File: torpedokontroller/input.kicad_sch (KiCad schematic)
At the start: 33 parts, among them IC8 TCAN3414DR, J2 653104124022, J8 USB_C_Receptacle_USB2.0_16P, U10 173950336, U4 WE-TVS-82400102, U8 BME280, U9 TPS26400PWP

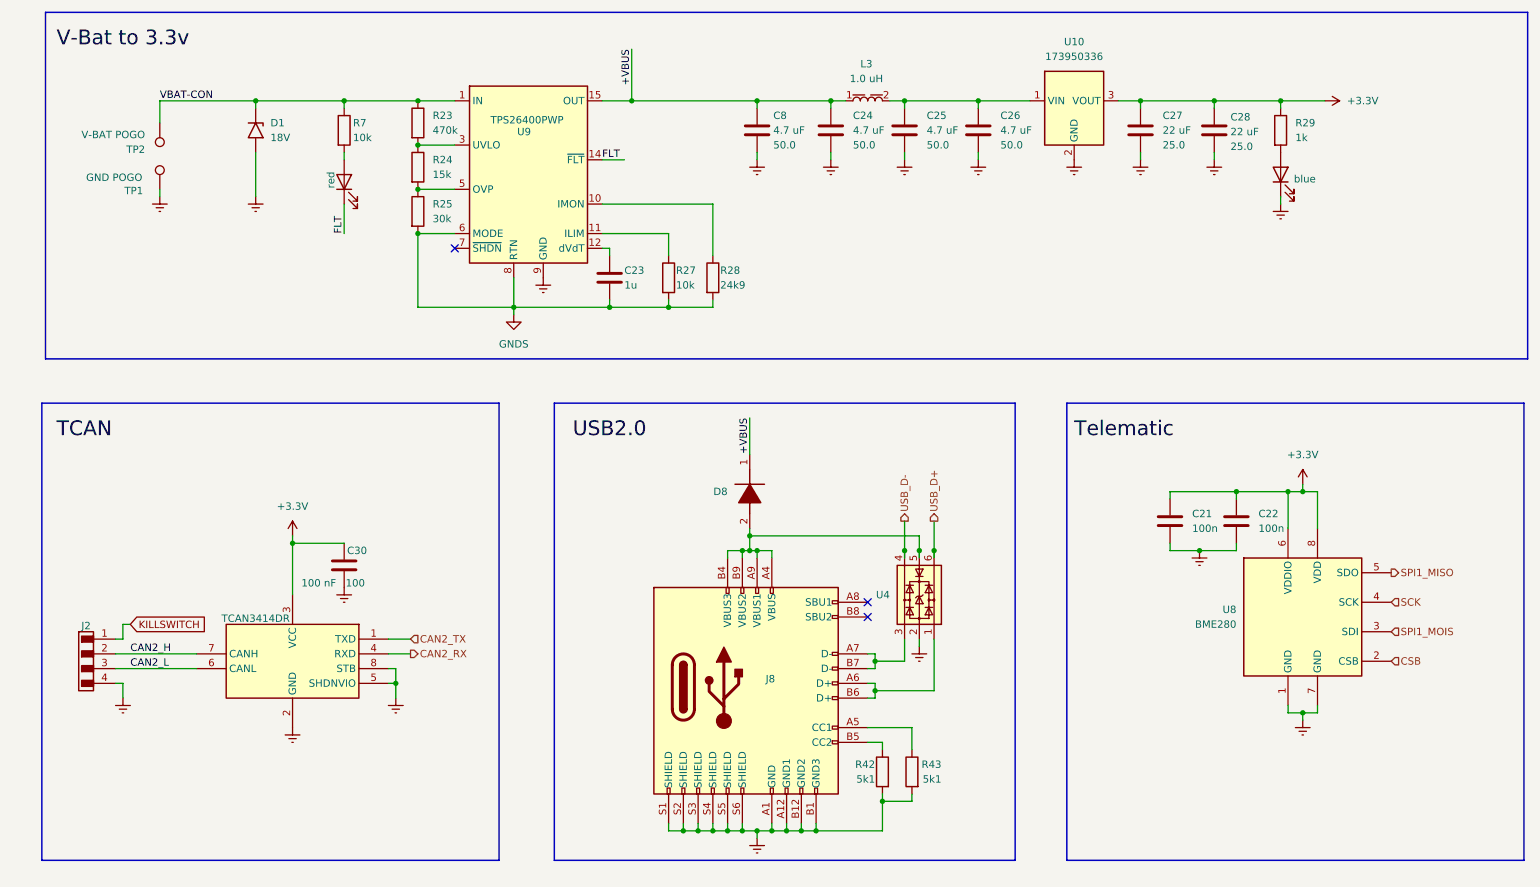
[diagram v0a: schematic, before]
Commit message: v 0.6
New MCU package
Added SWD, Rest and boot
Moved USB2.0 to MCU page
Other small changes
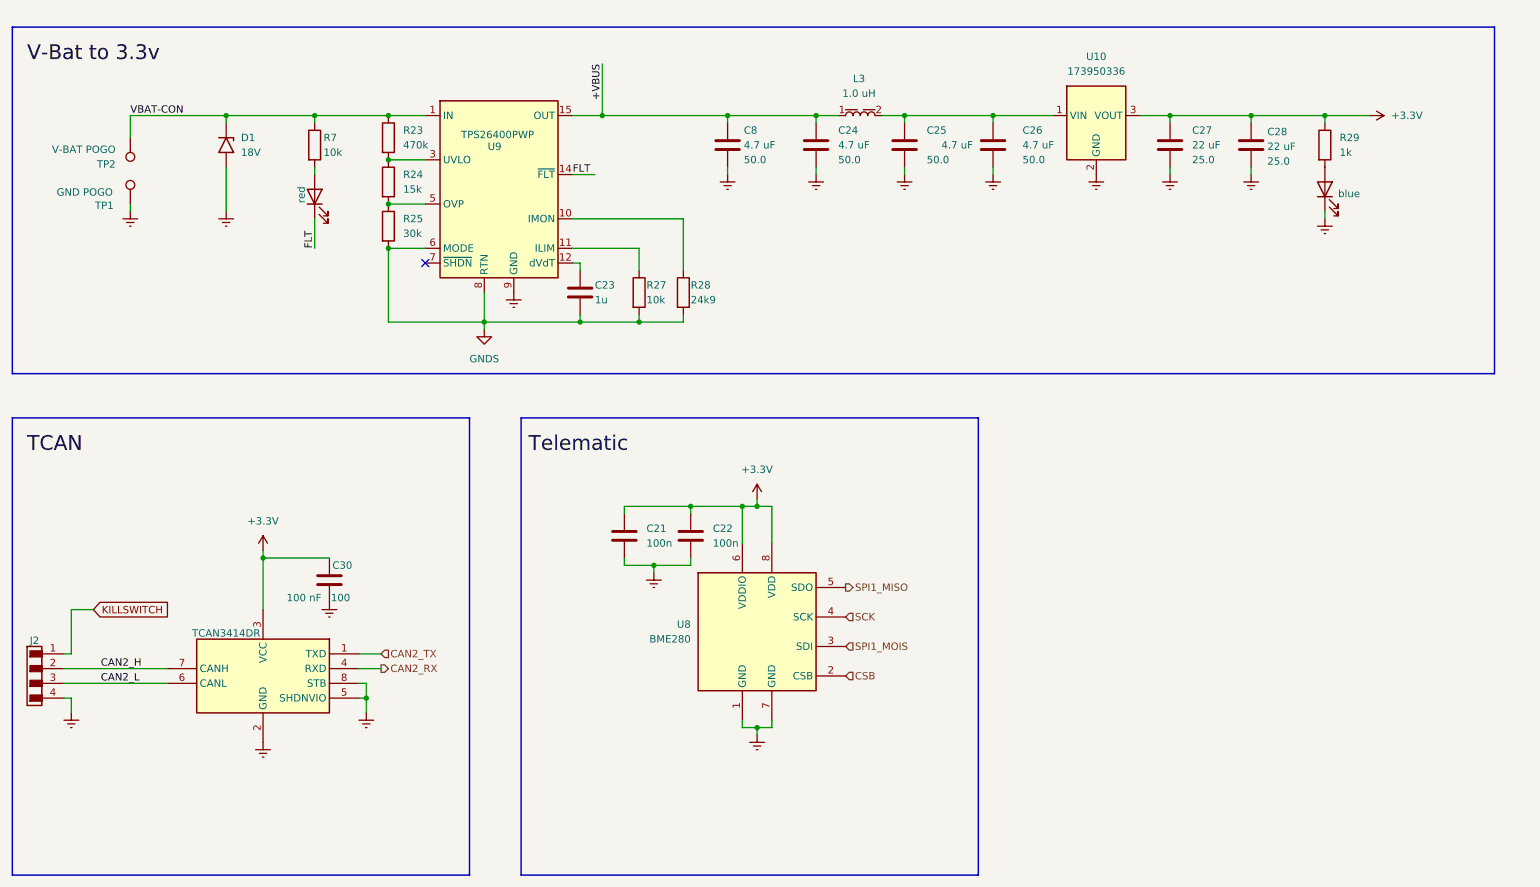
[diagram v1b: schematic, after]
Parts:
- removed D8: NSR0530HT1G, SOD2512X110N, symbol Schottky NSR0530HT1G:NSR0530HT1G
- removed J8: USB_C_Receptacle_USB2.0_16P, Connector_SMD_Wurth:J_Wurth_WR-USB_629722000214, symbol Connector:USB_C_Receptacle_USB2.0_16P
- removed R42, R43: 5k1, symbol Device:R
- removed U4: WE-TVS-82400102, Package_TO_SOT_SMD:SOT-23-6, symbol Power_Protection:WE-TVS-82400102
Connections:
- no-connect marks 3 -> 1
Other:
- moved on the sheet: C21, C22, C23, C24, C25, C26, C27, C28, C30, C8, D1, J2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
